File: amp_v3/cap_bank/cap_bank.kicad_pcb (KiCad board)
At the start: 2 copper layers, 31.2 x 88.4 mm, 8 parts, among them J1 Conn_01x02_Pin, J2 Conn_01x02_Pin

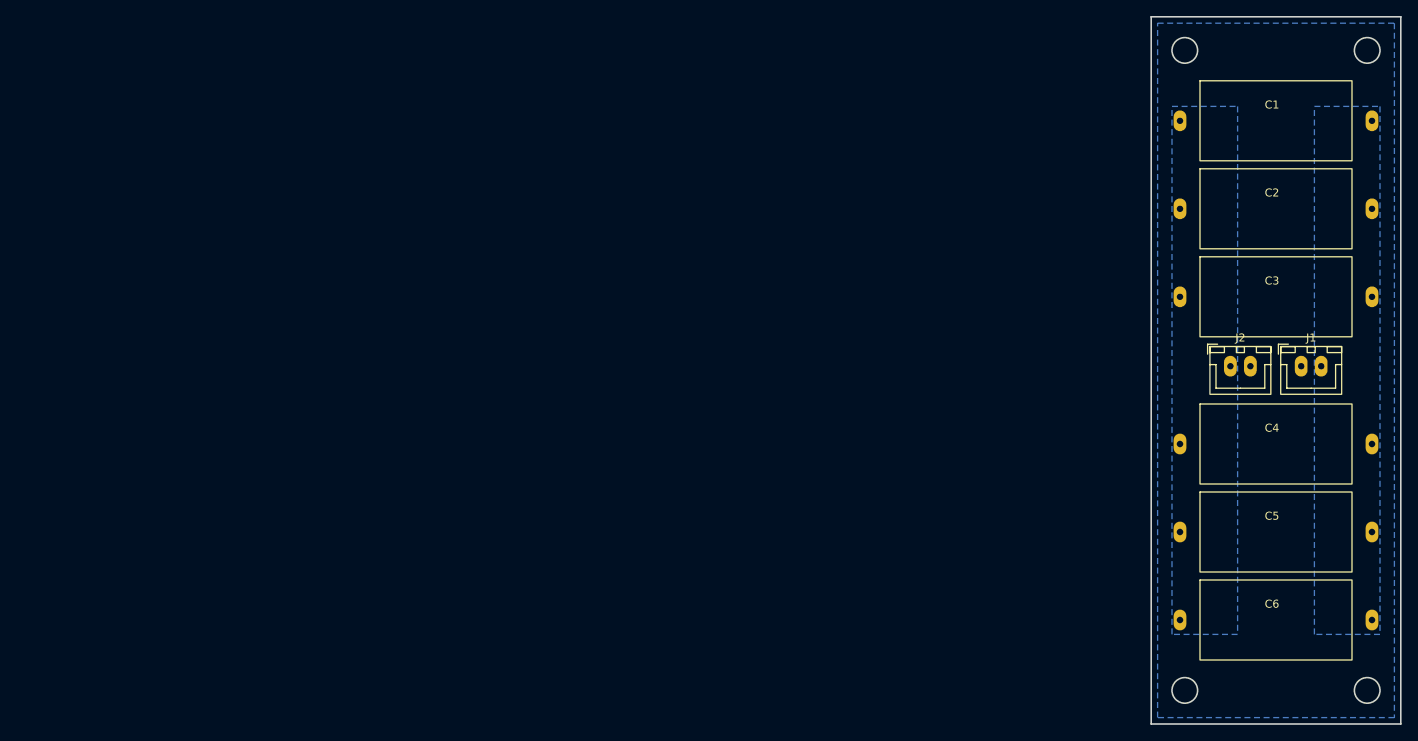
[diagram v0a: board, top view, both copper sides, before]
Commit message: updates
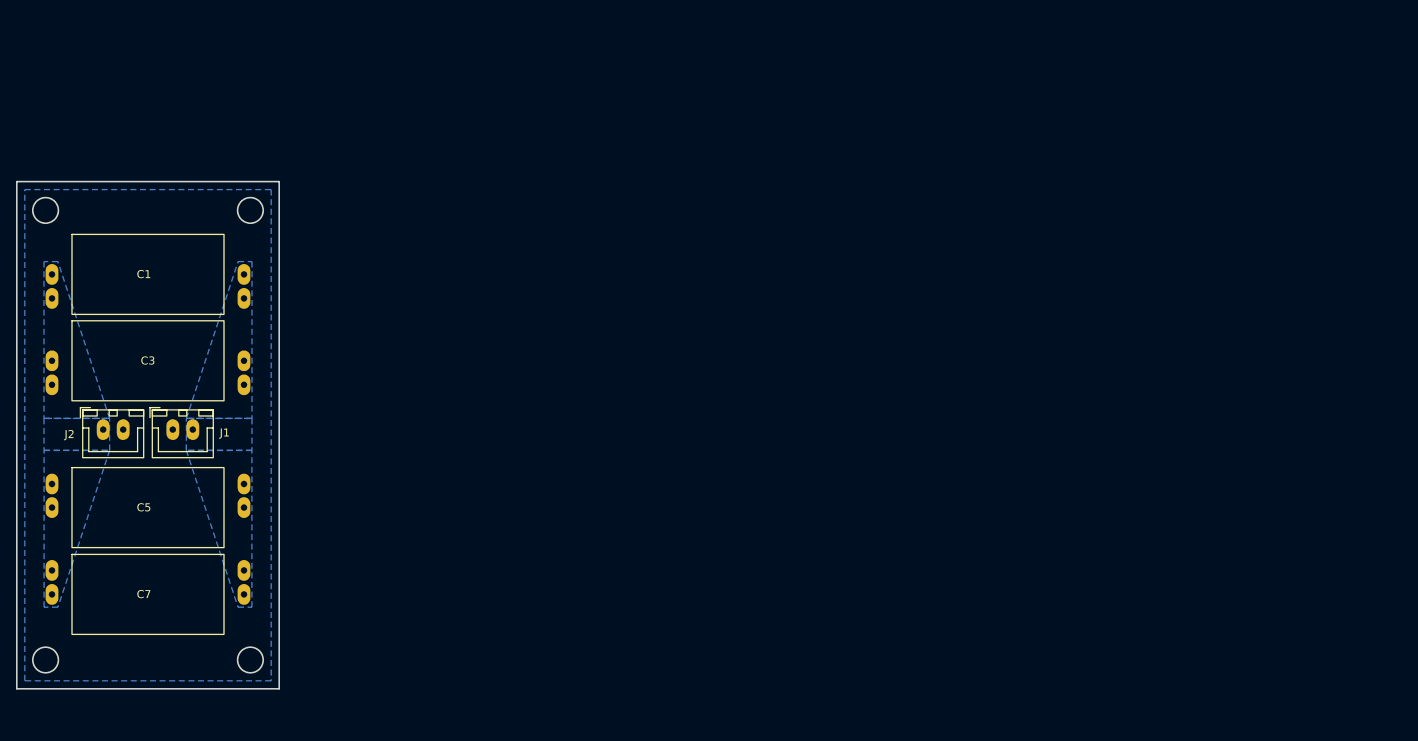
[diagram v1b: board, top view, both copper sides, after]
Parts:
- added C7: 1uF PP, Library:JFC, F.Cu at (33.3, 79.8)
- added C8: 1uF PP, Library:JFC, B.Cu at (33.3, 76.8)
- C1, C3, C5: value C -> 1uF PP
- C2, C4, C6: value C -> 1uF PP; moved to B.Cu
- moved C1 142.3 mm to (33.3, 39.8)
- moved C6 142.0 mm to (33.3, 66.0)
- moved C2 141.4 mm to (33.3, 42.8)
- moved J1 141.3 mm to (48.4, 59.1)
- moved C3 141.2 mm to (33.3, 50.5)
- moved C4 141.2 mm to (33.3, 53.5)
- moved J2 141.1 mm to (39.7, 59.1)
- moved C5 141.0 mm to (33.3, 68.9)
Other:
- board size 31.2 x 88.4 mm -> 32.8 x 63.4 mm
